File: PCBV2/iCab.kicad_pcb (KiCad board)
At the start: 2 copper layers, 58.4 x 90.2 mm, 95 parts, among them J1 S5, J10 D1, J11 D2, J12 D3, J13 D4, J14 D5, J2 S4, J5 S3, J6 S2, J8 S1, Q1 IRFZ44, Q2 IRFZ44, Q3 IRFZ44, Q4 IRFZ44, Q5 IRFZ44, U1 Output, U2 PIC18F2550, U3 Output, U4 L7805

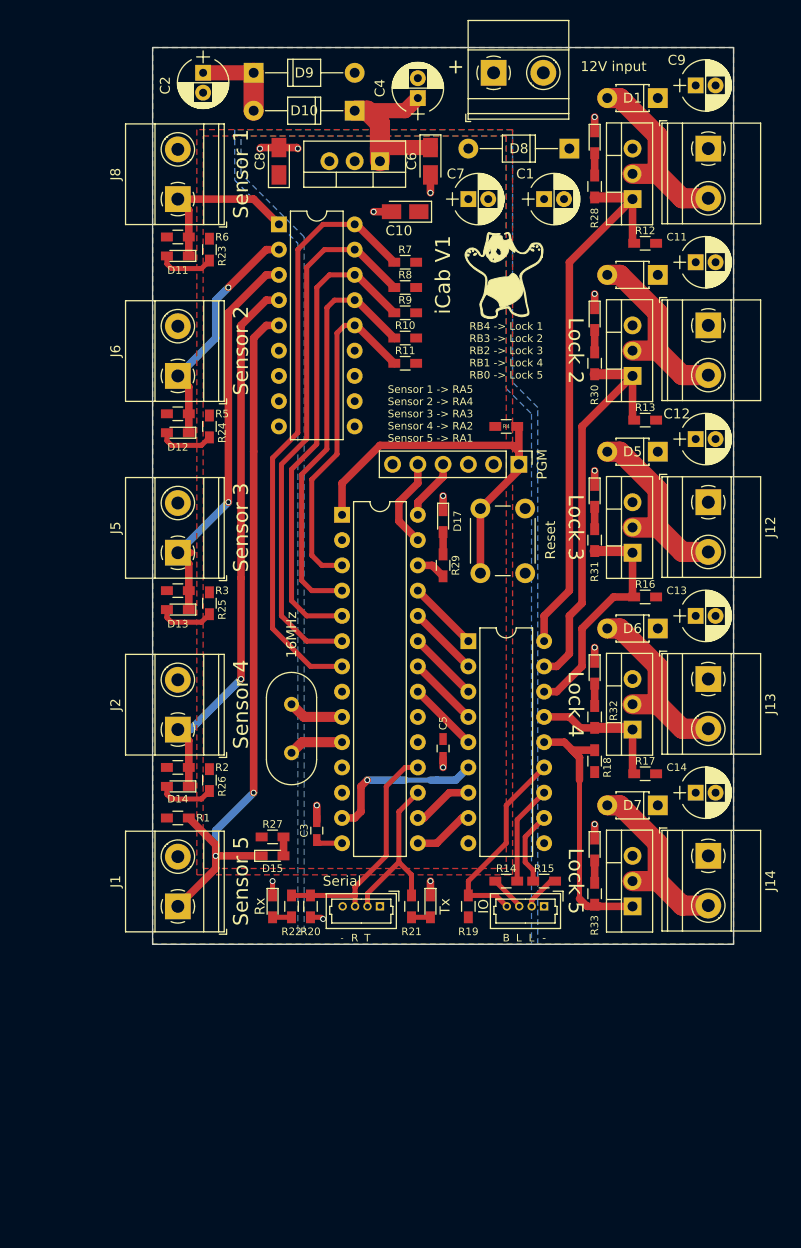
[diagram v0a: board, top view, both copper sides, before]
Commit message: pcb2
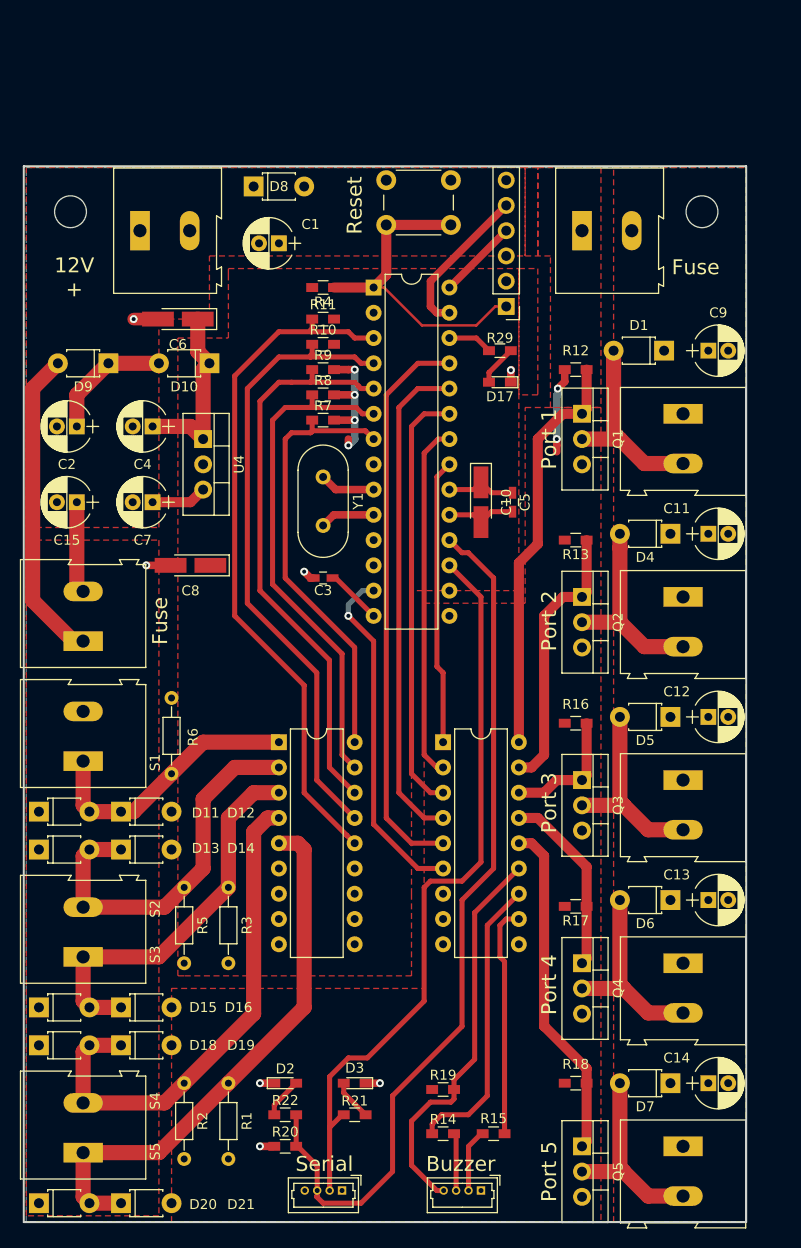
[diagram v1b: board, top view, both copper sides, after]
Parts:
- removed 12V input: 12V, TerminalBlock_Phoenix:TerminalBlock_Phoenix_MKDS-1,5-2_1x02_P5.00mm_Horizontal
- removed 16MHz: Crystal, Crystals:Crystal_HC49-U_Vertical
- removed G***: LOGO, panda:LOGO3
- removed G***: LOGO, KiCadLogos:galenus80_50
- removed IO: OUT, Connectors_Molex:Molex_PicoBlade_53047-0410_04x1.25mm_Straight
- removed J6: S2, TerminalBlock_Phoenix:TerminalBlock_Phoenix_MKDS-1,5-2_1x02_P5.00mm_Horizontal
- removed PGM: PGM, Pin_Headers:Pin_Header_Straight_1x06_Pitch2.54mm
- removed R23, R24, R25, R26, R27: 511, Resistors_SMD:R_0603_HandSoldering
- removed R28, R30, R31, R32, R33: 1.2k, Resistors_SMD:R_0603_HandSoldering
- removed Reset: SW_Push, Buttons_Switches_THT:SW_PUSH_6mm
- removed Rx, Tx: LED, LEDs:LED_0603_HandSoldering
- removed Serial: SERIAL, Connectors_Molex:Molex_PicoBlade_53047-0410_04x1.25mm_Straight
- added ?: , , F.Cu at (72.1, 104.1)
- added C15: 10µ, Capacitors_ThroughHole:CP_Radial_D5.0mm_P2.00mm, F.Cu at (64.8, 77.5)
- added D2: LED, LEDs:LED_0603_HandSoldering, F.Cu at (85.7, 135.9)
- added D3: LED, LEDs:LED_0603_HandSoldering, F.Cu at (92.7, 135.9)
- added H1: MountingHole, Mounting_Holes:MountingHole_3.2mm_M3, F.Cu at (64.1, 48.3)
- added H2: MountingHole, Mounting_Holes:MountingHole_3.2mm_M3, F.Cu at (127.6, 48.3)
- added J15: S5, Terminal_Blocks:TerminalBlock_Altech_AK300-2_P5.00mm, F.Cu at (115.6, 50.2)
- added J3: PGM, Pin_Headers:Pin_Header_Straight_1x06_Pitch2.54mm, F.Cu at (108.0, 57.8)
- added J4: SERIAL, Connectors_Molex:Molex_PicoBlade_53047-0410_04x1.25mm_Straight, F.Cu at (91.4, 146.7)
- added J7: OUT, Connectors_Molex:Molex_PicoBlade_53047-0410_04x1.25mm_Straight, F.Cu at (105.4, 146.7)
- added J9: 12V, Terminal_Blocks:TerminalBlock_Altech_AK300-2_P5.00mm, F.Cu at (71.1, 50.2)
- added SW1: SW_Push, Buttons_Switches_ThroughHole:SW_PUSH_6mm, F.Cu at (95.9, 45.1)
- added Y1: Crystal, Crystals:Crystal_HC49-U_Vertical, F.Cu at (89.5, 74.9)
- C1, C11, C12, C13, C14, C2, C4, C7, C9: footprint Capacitors_THT:CP_Radial_D5.0mm_P2.00mm -> Capacitors_ThroughHole:CP_Radial_D5.0mm_P2.00mm
- C10, C6, C8: footprint Capacitors_Tantalum_SMD:CP_Tantalum_Case-A_EIA-3216-18_Reflow -> Capacitors_Tantalum_SMD:CP_Tantalum_Case-A_EIA-3216-18_Hand
- D1, D4, D5, D6, D7: footprint Diodes_THT:D_T-1_P5.08mm_Horizontal -> Diodes_ThroughHole:D_T-1_P5.08mm_Horizontal
- D10, D8, D9: footprint Diodes_THT:D_T-1_P10.16mm_Horizontal -> Diodes_ThroughHole:D_T-1_P5.08mm_Horizontal
- D11, D12, D13, D14, D15, D16, D18, D19, D20, D21: value LED -> D; footprint LEDs:LED_0603_HandSoldering -> Diodes_ThroughHole:D_T-1_P5.08mm_Horizontal
- J1, J10, J11, J12, J13, J14, J2, J5: footprint TerminalBlock_Phoenix:TerminalBlock_Phoenix_MKDS-1,5-2_1x02_P5.00mm_Horizontal -> Terminal_Blocks:TerminalBlock_Altech_AK300-2_P5.00mm
- J8: value S1 -> S5; footprint TerminalBlock_Phoenix:TerminalBlock_Phoenix_MKDS-1,5-2_1x02_P5.00mm_Horizontal -> Terminal_Blocks:TerminalBlock_Altech_AK300-2_P5.00mm
- Q1, Q2, Q3, Q4, Q5, U4: footprint TO_SOT_Packages_THT:TO-220_Vertical -> TO_SOT_Packages_THT:TO-220-3_Vertical
- R1, R2, R3, R5, R6: value 10k -> 100k; footprint Resistors_SMD:R_0603_HandSoldering -> Resistors_ThroughHole:R_Axial_DIN0204_L3.6mm_D1.6mm_P7.62mm_Horizontal
- moved D16 99.2 mm to (69.2, 128.3), turned to 0 degrees
- moved D18 92.0 mm to (61.0, 132.1), turned to 0 degrees
- moved D20 77.3 mm to (61.0, 148.0), turned to 0 degrees
- moved D19 72.9 mm to (69.2, 132.1), turned to 0 degrees
- moved D21 59.4 mm to (69.2, 148.0), turned to 0 degrees
- moved D11 57.6 mm to (61.0, 108.6), turned to 0 degrees
- moved R6 54.0 mm to (74.3, 104.8), turned to 90 degrees
- moved U1 52.1 mm to (85.1, 101.6)
- moved R5 47.6 mm to (75.6, 116.2), turned to 270 degrees
- moved J8 45.5 mm to (65.4, 91.4)
- moved C7 44.0 mm to (72.4, 77.5), turned to 180 degrees
- moved C4 42.4 mm to (72.4, 69.8), turned to 180 degrees
- moved C8 41.6 mm to (76.2, 83.8), turned to 180 degrees
- moved D12 38.5 mm to (69.2, 108.6), turned to 0 degrees
- moved C2 37.8 mm to (64.8, 69.8), turned to 180 degrees
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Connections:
- C11 pad 1: +12V -> Net-(C11-Pad1)
- C12 pad 1: +12V -> Net-(C11-Pad1)
- C13 pad 1: +12V -> Net-(C11-Pad1)
- C14 pad 1: +12V -> Net-(C11-Pad1)
- C9 pad 1: +12V -> Net-(C11-Pad1)
- D1 pad 1: +12V -> Net-(C11-Pad1)
- D11 pad 1: /SI1 -> Net-(C15-Pad1)
- D11 pad 2: Net-(D11-Pad2) -> /SI1
- D12 pad 1: /SI2 -> /SI1
- D12 pad 2: Net-(D12-Pad2) -> GND
- D13 pad 1: /SI3 -> Net-(C15-Pad1)
- D13 pad 2: Net-(D13-Pad2) -> /SI2
- D14 pad 1: /SI4 -> /SI2
- D14 pad 2: Net-(D14-Pad2) -> GND
- D15 pad 1: /SI5 -> Net-(C15-Pad1)
- D15 pad 2: Net-(D15-Pad2) -> /SI3
- D16 pad 1: GND -> /SI3
- D16 pad 2: Net-(D16-Pad2) -> GND
- D18 pad 1: GND -> Net-(C15-Pad1)
- D18 pad 2: Net-(D18-Pad2) -> /SI4
- D19 pad 1: GND -> /SI4
- D19 pad 2: Net-(D19-Pad2) -> GND
- D20 pad 1: GND -> Net-(C15-Pad1)
- D20 pad 2: Net-(D20-Pad2) -> /SI5
- D21 pad 1: GND -> /SI5
- D21 pad 2: Net-(D21-Pad2) -> GND
- D4 pad 1: +12V -> Net-(C11-Pad1)
- D5 pad 1: +12V -> Net-(C11-Pad1)
- D6 pad 1: +12V -> Net-(C11-Pad1)
- D7 pad 1: +12V -> Net-(C11-Pad1)
- J1 pad 2: GND -> /SI4
- J10 pad 1: +12V -> Net-(C11-Pad1)
- J11 pad 1: +12V -> Net-(C11-Pad1)
- J12 pad 1: +12V -> Net-(C11-Pad1)
- J13 pad 1: +12V -> Net-(C11-Pad1)
- J14 pad 1: +12V -> Net-(C11-Pad1)
- J2 pad 1: /SI4 -> /SI3
- J2 pad 2: GND -> /SI2
- J5 pad 1: /SI3 -> /SI1
- J5 pad 2: GND -> Net-(C15-Pad1)
- J8 pad 1: /SI1 -> +12V
- J8 pad 2: GND -> Net-(C15-Pad1)
- R1 pad 2: +12V -> GND
- R2 pad 2: +12V -> GND
- R3 pad 2: +12V -> GND
- R5 pad 2: +12V -> GND
- R6 pad 2: +12V -> GND
- U1 pad 11: (no net) -> Net-(U1-Pad11)
- U1 pad 12: (no net) -> Net-(U1-Pad12)
- U1 pad 13: (no net) -> Net-(U1-Pad13)
- U1 pad 6: (no net) -> Net-(U1-Pad6)
- U1 pad 7: (no net) -> Net-(U1-Pad7)
- U1 pad 8: (no net) -> Net-(U1-Pad8)
- U2 pad 11: (no net) -> Net-(U2-Pad11)
- U2 pad 12: (no net) -> Net-(U2-Pad12)
- U2 pad 15: /L1 -> Net-(U2-Pad15)
- U2 pad 16: /L2 -> Net-(U2-Pad16)
- U2 pad 2: (no net) -> Net-(U2-Pad2)
- U2 pad 21: /PI5 -> /PI1
- U2 pad 22: /PI4 -> /PI2
- U2 pad 24: /PI2 -> /PI4
- U2 pad 25: /PI1 -> /PI5
- U3 pad 7: /L2 -> Net-(U3-Pad7)
- U3 pad 8: /L1 -> Net-(U3-Pad8)
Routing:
- net /SER_RX: track 23.9 -> 88.4 mm
- net /SER_TX: track 17.4 -> 75.4 mm
- net /PI5: track 7.18 -> 57.0 mm
- net /PI4: track 7.18 -> 50.1 mm
- net +12V: track 0.00 -> 40.3 mm, vias 0 -> 2
- net /PI3: track 7.18 -> 43.2 mm
- net /SO1: track 34.7 -> 69.4 mm
- net /PI2: track 7.18 -> 35.9 mm
- net +5V: track 0.00 -> 27.4 mm, vias 0 -> 4
- net /PI1: track 7.18 -> 28.7 mm
- net /SO2: track 41.8 -> 63.3 mm
- net /Buzzer: track 20.4 -> 39.8 mm
- net Net-(R14-Pad1): track 10.0 -> 29.3 mm
- net /PWM: track 16.9 -> 35.1 mm
- net /SI5: track 72.9 -> 55.5 mm, vias 2 -> 0
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- added copper zone on F.Cu, net Net-(C11-Pad1)
- added copper zone on F.Cu, net Net-(C15-Pad1)
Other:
- board size 58.4 x 90.2 mm -> 72.6 x 106.2 mm
- net class Default: via_dia 0.6 -> 0.8
- board text added: "12V +"
- board text added: "Buzzer"
- board text added: "Fuse"
- board text added: "Port 1"
- board text added: "Port 2"
- board text added: "Port 3"
- board text added: "Port 4"
- board text added: "Port 5"
- board text added: "Reset"
- board text added: "S1"
- board text added: "S2"
- board text added: "S3"
- board text added: "S4"
- board text added: "S5"
- board text added: "Serial"
- board text removed: "+"
- board text removed: "-"
- board text removed: "B"
- board text removed: "L"
- board text removed: "Lock 2"
- board text removed: "Lock 3"
- board text removed: "Lock 4"
- board text removed: "Lock 5"
- board text removed: "R"
- board text removed: "RB4 -> Lock 1 RB3 -> Lock 2 RB2 -> Lock 3 RB1 -> Lock 4 RB0 -> Lock 5"
- board text removed: "Sensor 1"
- board text removed: "Sensor 1 -> RA5 Sensor 2 -> RA4 Sensor 3 -> RA3 Sensor 4 -> RA2 Sensor 5 -> RA1"
- board text removed: "Sensor 2"
- board text removed: "Sensor 3"
- board text removed: "Sensor 4"
- board text removed: "Sensor 5"
- board text removed: "T"
- board text removed: "iCab V1"
